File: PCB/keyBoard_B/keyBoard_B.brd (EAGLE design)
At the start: 169.5 x 134.6 mm, 284 parts

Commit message: .
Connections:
- net N$393 renamed G6C
- net N$394 renamed G6B
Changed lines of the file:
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@@
 <?xml version="1.0" encoding="utf-8"?>
 <!DOCTYPE eagle SYSTEM "eagle.dtd">
-<eagle version="6.3">
+<eagle version="6.4">
 <drawing>
 <settings>
@@
 <wire x1="69.05625" y1="106.045" x2="69.05625" y2="113.18875" width="0.4064" layer="21" style="shortdash"/>
 <wire x1="69.05625" y1="113.18875" x2="61.75375" y2="120.3325" width="0.4064" layer="21" style="shortdash"/>
-<dimension x1="31.115" y1="150.495" x2="30.95625" y2="15.875" x3="24.844375" y3="83.185" layer="21" dtype="vertical"/>
+<dimension x1="31.115" y1="150.495" x2="30.95625" y2="15.875" x3="24.844375" y3="83.185" textsize="3.5" layer="21" dtype="vertical"/>
 <circle x="169.38625" y="41.275" radius="2.5" width="0.254" layer="20"/>
-<dimension x1="25.4" y1="15.08125" x2="30.63875" y2="15.08125" x3="28.019375" y3="10.31875" layer="21" dtype="horizontal"/>
-<dimension x1="24.13" y1="40.9575" x2="22.06625" y2="15.875" x3="15.954375" y3="28.41625" layer="21" dtype="vertical"/>
+<dimension x1="25.4" y1="15.08125" x2="30.63875" y2="15.08125" x3="28.019375" y3="10.31875" textsize="3.5" layer="21" dtype="horizontal"/>
+<dimension x1="24.13" y1="40.9575" x2="22.06625" y2="15.875" x3="15.954375" y3="28.41625" textsize="3.5" layer="21" dtype="vertical"/>
 <wire x1="25.4" y1="22.38375" x2="25.4" y2="19.05" width="0.2" layer="20"/>
 <wire x1="25.4" y1="19.05" x2="28.575" y2="15.875" width="0.2" layer="20" curve="90"/>
 <wire x1="30.95625" y1="19.05" x2="34.13125" y2="15.875" width="0.2" layer="20" curve="90"/>
-<dimension x1="30.95625" y1="150.97125" x2="194.945" y2="149.86" x3="112.950625" y3="153.67" layer="21" dtype="horizontal"/>
-<dimension x1="25.4" y1="7.14375" x2="194.945" y2="14.12875" x3="110.1725" y3="4.92125" layer="21" dtype="horizontal"/>
+<dimension x1="30.95625" y1="150.97125" x2="194.945" y2="149.86" x3="112.950625" y3="153.67" textsize="3.5" layer="21" dtype="horizontal"/>
+<dimension x1="25.4" y1="7.14375" x2="194.945" y2="14.12875" x3="110.1725" y3="4.92125" textsize="3.5" layer="21" dtype="horizontal"/>
 </plain>
 <attributes>
@@
 <wire x1="175.895" y1="108.74375" x2="173.83125" y2="112.7125" width="0.6096" layer="16"/>
 </signal>
-<signal name="N$393">
+<signal name="G6C">
 <contactref element="JA67" pad="2"/>
 <contactref element="JA67B" pad="2"/>
@@
 <wire x1="177.32375" y1="106.52125" x2="173.7995" y2="106.52125" width="0.6096" layer="16"/>
 </signal>
-<signal name="N$394">
+<signal name="G6B">
 <contactref element="J84" pad="1"/>
 <contactref element="J85" pad="2"/>

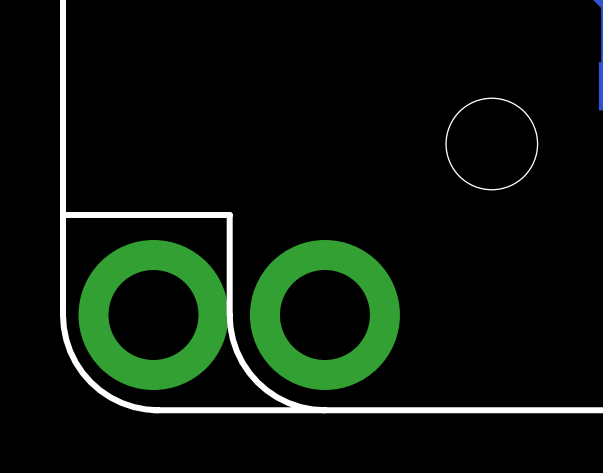
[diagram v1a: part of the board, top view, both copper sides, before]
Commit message: .
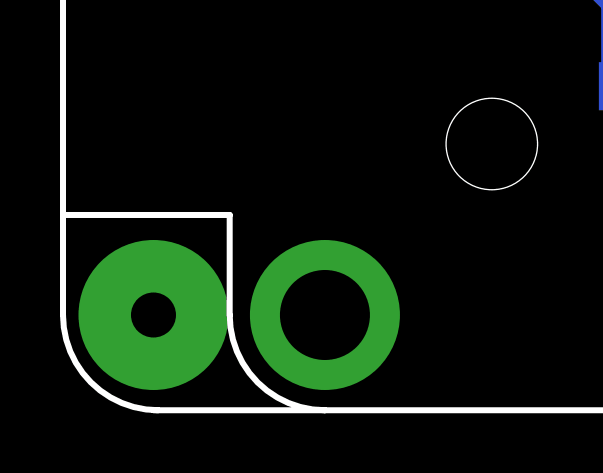
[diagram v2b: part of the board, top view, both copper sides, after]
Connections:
- net N$367 renamed G11
- net N$375 renamed G14
- net N$376 renamed G13
- net N$377 renamed G12
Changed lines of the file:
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@@
 <setting verticaltext="up"/>
 </settings>
-<grid distance="12.5" unitdist="mil" unit="mil" style="lines" multiple="1" display="yes" altdistance="0.025" altunitdist="inch" altunit="inch"/>
+<grid distance="12.5" unitdist="mil" unit="mm" style="lines" multiple="1" display="yes" altdistance="0.025" altunitdist="inch" altunit="inch"/>
 <layers>
 <layer number="1" name="Top" color="4" fill="1" visible="yes" active="yes"/>
@@
 </signal>
 <signal name="N$11">
-<via x="28.41625" y="19.05" extent="1-16" drill="3" diameter="5"/>
+<via x="28.41625" y="19.05" extent="1-16" drill="1.5" diameter="5"/>
 </signal>
 <signal name="N$407">
@@
 <wire x1="73.18375" y1="126.2765" x2="73.81875" y2="125.095" width="0.6096" layer="16"/>
 </signal>
-<signal name="N$367">
+<signal name="G11">
 <contactref element="2D2" pad="8"/>
 <contactref element="J69" pad="2"/>
@@
 <wire x1="78.89875" y1="125.095" x2="77.54025" y2="127.635" width="0.6096" layer="16"/>
 </signal>
-<signal name="N$375">
+<signal name="G14">
 <contactref element="J67" pad="1"/>
 <wire x1="38.89375" y1="121.92" x2="42.545" y2="125.57125" width="0.4064" layer="16"/>
@@
 <wire x1="64.61125" y1="129.54" x2="67.46875" y2="131.445" width="0.4064" layer="16"/>
 </signal>
-<signal name="N$376">
+<signal name="G13">
 <contactref element="J67" pad="2"/>
 <contactref element="J68" pad="1"/>
 <wire x1="71.82525" y1="131.445" x2="73.90725" y2="131.445" width="1.016" layer="16"/>
 </signal>
-<signal name="N$377">
+<signal name="G12">
 <contactref element="J68" pad="2"/>
 <contactref element="J69" pad="1"/>
